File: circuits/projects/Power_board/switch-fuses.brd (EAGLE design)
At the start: 75 x 50 mm, 22 parts

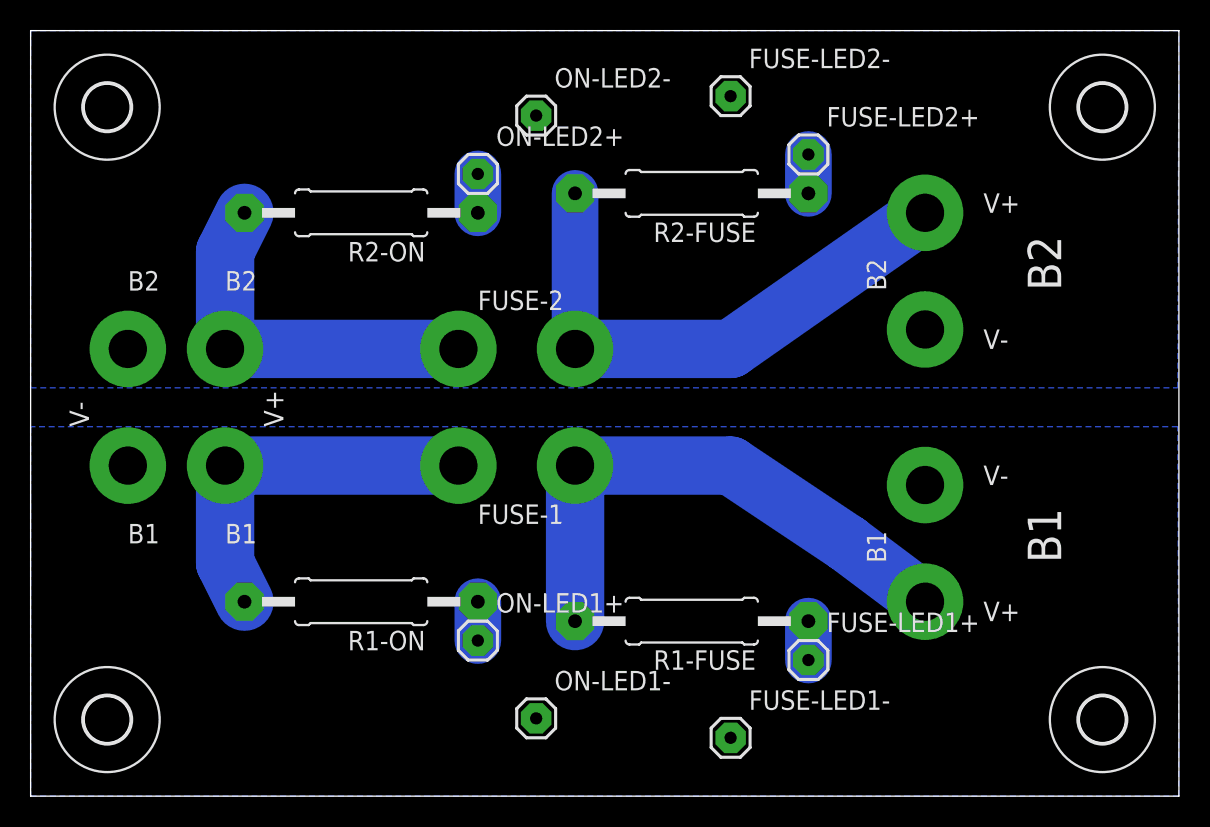
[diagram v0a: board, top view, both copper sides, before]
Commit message: new shit
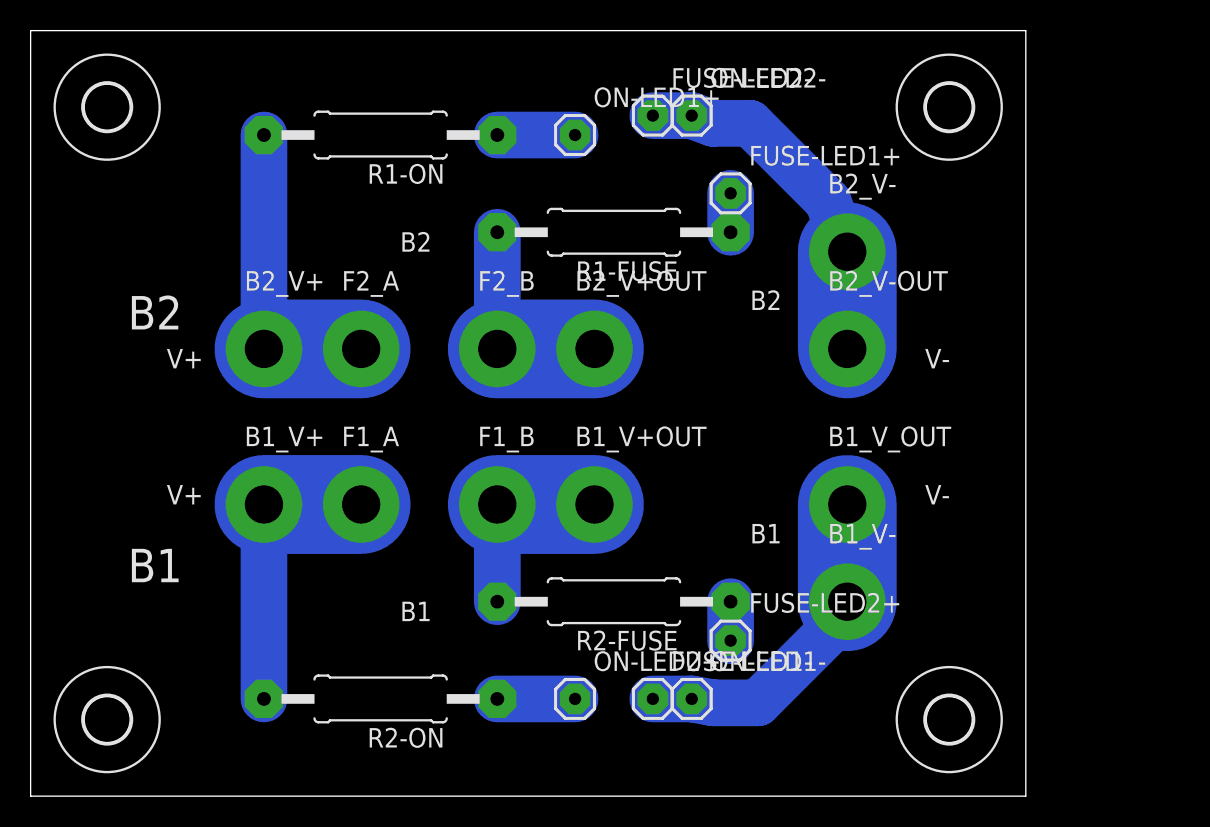
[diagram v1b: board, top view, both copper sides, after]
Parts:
- removed B1, B2, FUSE-1, FUSE-2, V+, V-: 2-HOLES2.5MM, parts:2-HOLE-2.5MM
- added B1_V+, B1_V+OUT, B1_V-, B1_V_OUT, B2_V+, B2_V+OUT, B2_V-, B2_V-OUT, F1_A, F1_B, F2_A, F2_B: 1-HOLE2.5MM, parts:1-HOLE-2.5MM
- moved ON-LED2+ 34.9 mm to (35.6, 6.35)
- moved ON-LED1+ 33.6 mm to (35.6, 43.2)
- moved FUSE-LED2+ 32.2 mm to (45.7, 10.2)
- moved R2-ON 31.8 mm to (22.9, 6.35)
- moved FUSE-LED1+ 30.9 mm to (45.7, 39.4)
- moved R1-ON 30.5 mm to (22.9, 43.2)
- moved R2-FUSE 27.1 mm to (38.1, 12.7)
- moved R1-FUSE 25.9 mm to (38.1, 36.8)
- moved ON-LED1- 10.2 mm to (43.2, 6.35)
- moved ON-LED2- 10.2 mm to (43.2, 44.5)
- moved U$2 10.0 mm to (60.0, 45.0)
- moved U$4 10.0 mm to (60.0, 5.00)
- moved FUSE-LED1- 5.68 mm to (40.6, 6.35)
- moved FUSE-LED2- 5.24 mm to (40.6, 44.5)
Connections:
- net V+1: now also B2_V+OUT.P$1, F2_B.P$1; no longer B1.1, FUSE-1.2
- net V+2: now also B1_V+OUT.P$1, F1_B.P$1; no longer B2.2, FUSE-2.2
- net V-1: now also B1_V-.P$1, B1_V_OUT.P$1; no longer B1.2, V-.1
- net V-2: now also B2_V-.P$1, B2_V-OUT.P$1; no longer B2.1, V-.2
- net VIN1: now also B1_V+.P$1, F1_A.P$1; no longer FUSE-2.1, V+.2
- net VIN2: now also B2_V+.P$1, F2_A.P$1; no longer FUSE-1.1, V+.1
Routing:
- net V+2: track 37.1 -> 12.7 mm
- net V-2: track 0.00 -> 23.5 mm
- net V-1: track 0.00 -> 22.3 mm
- net V+1: track 35.8 -> 14.0 mm
- net VIN1: track 24.4 -> 19.1 mm
- net VIN2: track 24.4 -> 20.3 mm
- net N$9: track 2.54 -> 5.08 mm
- net N$10: track 2.54 -> 5.08 mm
- removed copper zone on layer 16, net V-1
- removed copper zone on layer 16, net V-2
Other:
- board size 75 x 50 mm -> 65 x 50 mm
